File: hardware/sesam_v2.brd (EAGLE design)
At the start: 70 x 70 mm, 13 parts

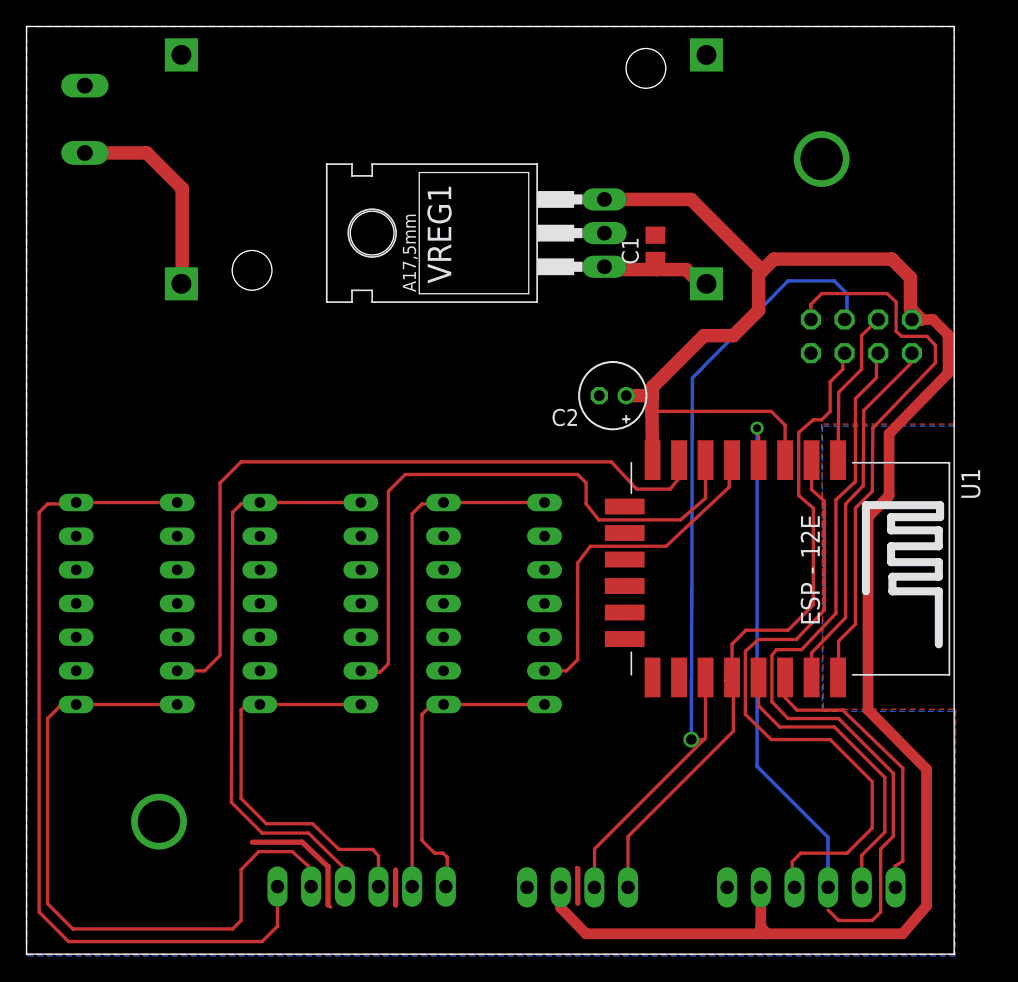
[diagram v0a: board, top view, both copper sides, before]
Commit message: minor tweaks of the board and change of display text size
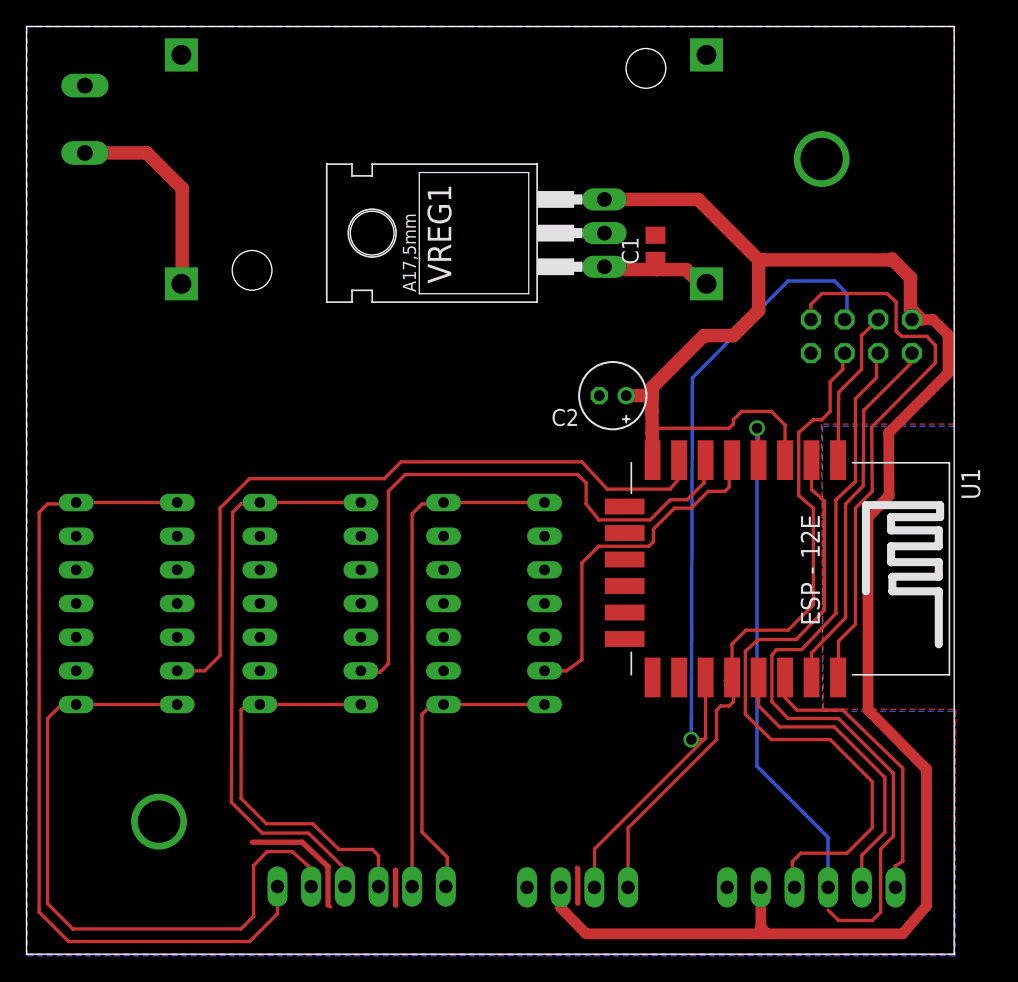
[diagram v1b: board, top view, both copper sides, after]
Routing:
- net GND: track 0.00 -> 15.0 mm
- net N$7: track 9.59 -> 0.00 mm
- net N$8: track 2.74 -> 0.00 mm
- net N$6: track 2.65 -> 0.00 mm
- net GPIO0: track 50.4 -> 51.7 mm
- net GPIO13: track 54.7 -> 53.6 mm
- net 3V3: track 149.1 -> 150.1 mm
- net GPIO12: track 45.8 -> 45.1 mm
- net N$14: track 63.3 -> 62.7 mm
